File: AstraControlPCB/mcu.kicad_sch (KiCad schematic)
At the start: 9 parts, among them U1 ESP32-S3-WROOM-1U-N8

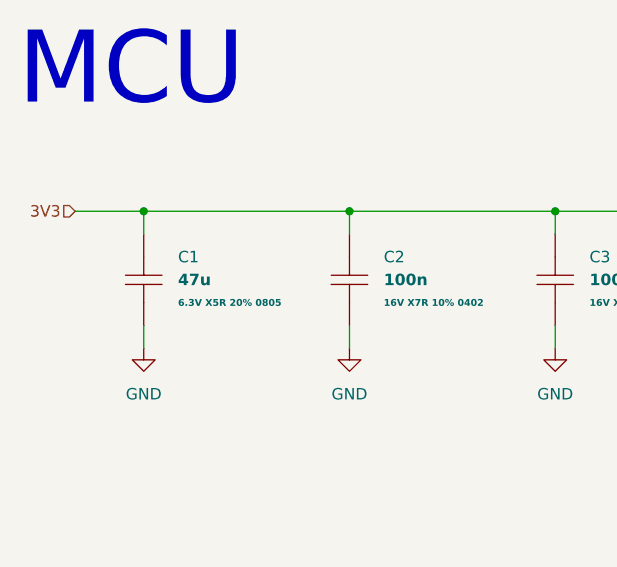
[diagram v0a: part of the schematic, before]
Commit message: Updated Pi filter
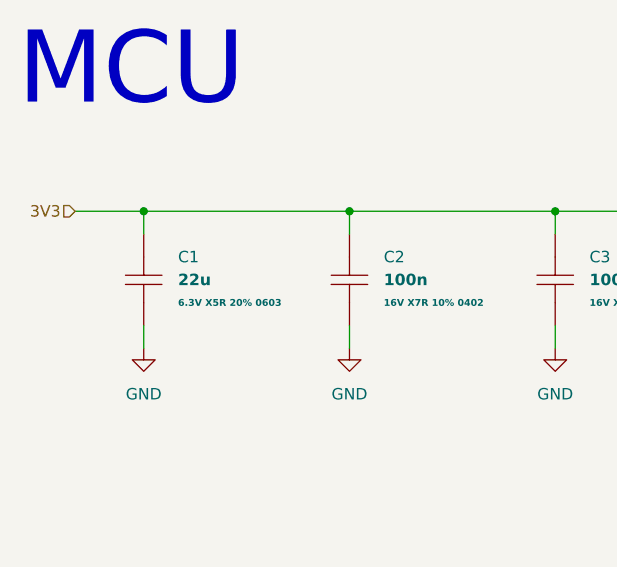
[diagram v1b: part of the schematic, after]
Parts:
- removed C1: 47u, LiveAstra:C_0805_2012Metric_Pad1.18x1.45mm_HandSolder, symbol LiveAstra:C_47u_X5R_0805
- added C1: 22u, LiveAstra:C_0603_1608Metric, symbol LiveAstra:C_22uF_X5R_0603
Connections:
- net 3V3: now also C1.2
- net GND: now also C1.1
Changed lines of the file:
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@@
+	)
+	(symbol
+		(lib_id "LiveAstra:C_22uF_X5R_0603")
+		(at 33.02 53.34 90)
+		(unit 1)
+		(exclude_from_sim no)
+		(in_bom yes)
+		(on_board yes)
+		(dnp no)
+		(fields_autoplaced yes)
+		(property "Reference" "C1"
+			(at 36.83 50.7999 90)
+			(effects
+				(font
+					(size 1.27 1.27)
+				)
+				(justify right)
+			)
+		)
+		(property "Value" "22u"
+			(at 36.83 53.34 90)
+			(effects
+				(font
+					(size 1.27 1.27)
+					(bold yes)
+				)
+				(justify right)
+			)
+		)
+		(property "Footprint" "LiveAstra:C_0603_1608Metric"
+			(at 41.91 53.34 0)
+			(effects
+				(font
+					(size 1.27 1.27)
+				)
+				(hide yes)
+			)
+		)
+		(property "Datasheet" "https://lcsc.com/product-detail/Multilayer-Ceramic-Capacitors-MLCC-SMD-SMT_SAMSUNG_CL10A226MQ8NRNC_22uF-226-20-6-3V_C59461.html"
+			(at 45.72 53.34 0)
+			(effects
+				(font
+					(size 1.27 1.27)
+				)
+				(hide yes)
+			)
+		)
+		(property "Description" "6.3V 22uF X5R ±20% 0603 Multilayer Ceramic Capacitors MLCC - SMD/SMT ROHS"
+			(at 38.1 53.34 0)
+			(effects
+				(font
+					(size 1.27 1.27)
+				)
+				(hide yes)
+			)
+		)
+		(property "LCSC Part" "C59461"
+			(at 49.53 53.34 0)
+			(effects
+				(font
+					(size 1.27 1.27)
+				)
+				(hide yes)
+			)
+		)
+		(property "Extra Values" "6.3V X5R 20% 0603"
+			(at 36.83 55.8799 90)
+			(effects
+				(font
+					(size 0.762 0.762)
+					(bold yes)
+				)
+				(justify right)
+			)
+		)
+		(property "MPN" "CL10A226MQ8NRNC"
+			(at 53.34 53.34 0)
+			(effects
+				(font
+					(size 1.27 1.27)
+				)
+				(hide yes)
+			)
+		)
+		(property "MFN" "Samsung Electro-Mechanics"
+			(at 57.15 53.34 0)
+			(effects
+				(font
+					(size 1.27 1.27)
+				)
+				(hide yes)
+			)
+		)
+		(pin "2"
+		)
+		(pin "1"
+		)
+		(instances
+			(project ""
+				(path "/9a751838-dce8-4d69-8a02-736625ac74e7/0db21d8e-3390-4d67-877f-0e5d98e37848/3087dd4a-2a8a-4df4-b1d8-8d4a2b3256a2"
+					(reference "C1")
+					(unit 1)
+				)
+			)
+		)
 	)
 	(symbol
@@
 					(unit 1)
 				)
-			)
-		)
-	)
-	(symbol
-		(lib_id "LiveAstra:C_47u_X5R_0805")
-		(at 33.02 53.34 90)
-		(unit 1)
-		(exclude_from_sim no)
-		(in_bom yes)
-		(on_board yes)
-		(dnp no)
-		(fields_autoplaced yes)
-		(property "Reference" "C1"
-			(at 36.83 50.7999 90)
-			(effects
-				(font
-					(size 1.27 1.27)
-				)
-				(justify right)
-			)
-		)
-		(property "Value" "47u"
-			(at 36.83 53.34 90)
-			(effects
-				(font
-					(size 1.27 1.27)
-					(bold yes)
-				)
-				(justify right)
-			)
-		)
-		(property "Footprint" "LiveAstra:C_0805_2012Metric_Pad1.18x1.45mm_HandSolder"
-			(at 41.91 53.34 0)
-			(effects
-				(font
-					(size 1.27 1.27)
-				)
-				(hide yes)
-			)
-		)
-		(property "Datasheet" "https://lcsc.com/product-detail/Multilayer-Ceramic-Capacitors-MLCC-SMD-SMT_SAMSUNG_CL21A476MQYNNNE_47uF-476-20-6-3V_C16780.html"
-			(at 45.72 53.34 0)
-			(effects
-				(font
-					(size 1.27 1.27)
-				)
-				(hide yes)
-			)
-		)
-		(property "Description" "6.3V 47uF X5R ±20% 0805 Multilayer Ceramic Capacitors MLCC - SMD/SMT ROHS"
-			(at 38.1 53.34 0)
-			(effects
-				(font
-					(size 1.27 1.27)
-				)
-				(hide yes)
-			)
-		)
-		(property "LCSC Part" "C16780"
-			(at 49.53 53.34 0)
-			(effects
-				(font
-					(size 1.27 1.27)
-				)
-				(hide yes)
-			)
-		)
-		(property "Extra Values" "6.3V X5R 20% 0805"
-			(at 36.83 55.8799 90)
-			(effects
-				(font
-					(size 0.762 0.762)
-					(bold yes)
-				)
-				(justify right)
-			)
-		)
-		(property "MFN" "Samsung Electro-Mechanics"
-			(at 53.34 53.34 0)
-			(effects
-				(font
-					(size 1.27 1.27)
-				)
-				(hide yes)
-			)
-		)
-		(property "MPN" "CL21A476MQYNNNE"
-			(at 53.34 53.34 0)
-			(effects
-				(font
-					(size 1.27 1.27)
-				)
-				(hide yes)
-			)
-		)
-		(pin "1"
-		)
-		(pin "2"
-		)
-		(instances
-			(project ""
-				(path "/9a751838-dce8-4d69-8a02-736625ac74e7/0db21d8e-3390-4d67-877f-0e5d98e37848/3087dd4a-2a8a-4df4-b1d8-8d4a2b3256a2"
-					(reference "C1")
-					(unit 1)
-				)
